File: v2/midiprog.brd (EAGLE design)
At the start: 99.1 x 78.7 mm, 56 parts, among them IC1 PIC18F4550_40, IC2 TPIC6B596N, IC4 TPIC6B596N, Q2 2N2222A, Q3 2N2222A, Q4 2N2222A, Q5 8MHz

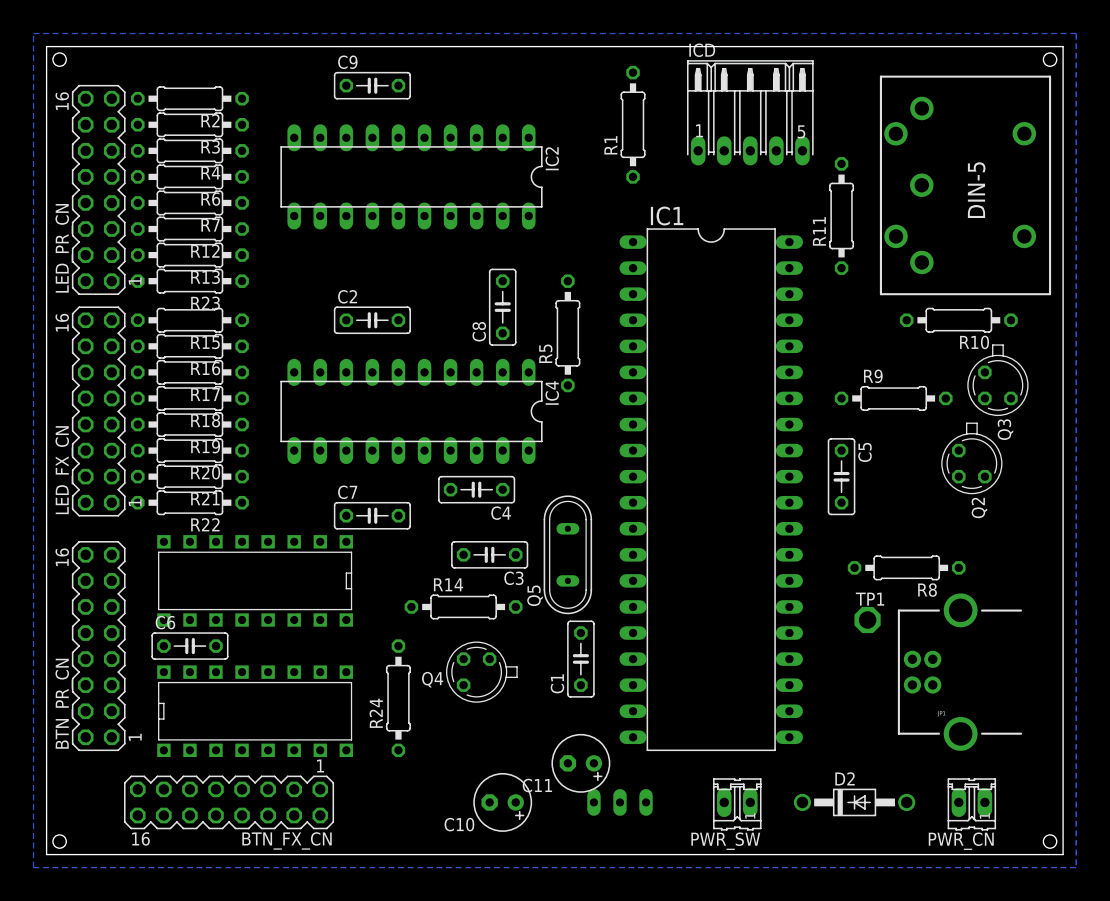
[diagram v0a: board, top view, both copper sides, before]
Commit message: Cleaning up board.
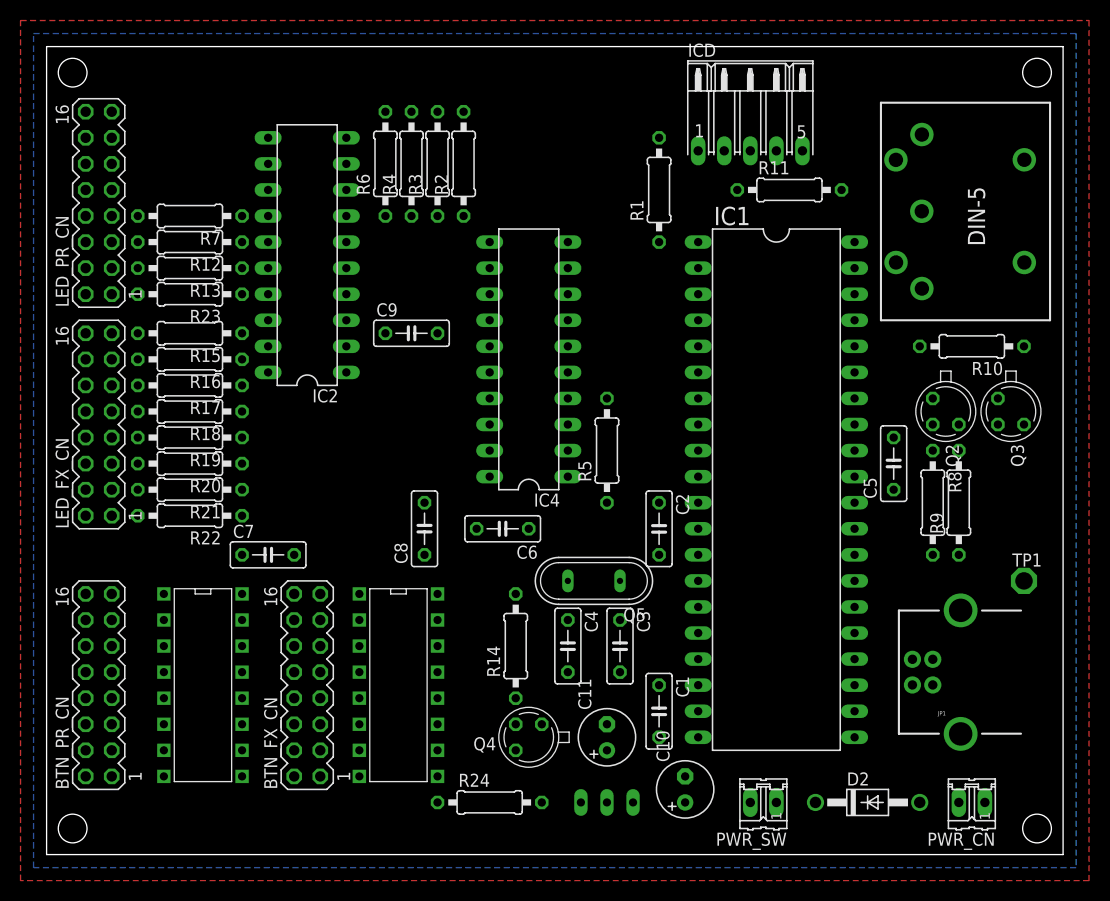
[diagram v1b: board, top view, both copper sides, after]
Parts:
- moved C2 34.5 mm to (59.7, 31.8), turned to 270 degrees
- moved C6 32.6 mm to (44.5, 31.8), turned to 180 degrees
- moved R2 27.4 mm to (40.6, 67.3), turned to 90 degrees
- moved C9 24.4 mm to (35.6, 50.8)
- moved R3 24.4 mm to (38.1, 67.3), turned to 90 degrees
- moved C8 22.9 mm to (36.8, 31.8)
- moved R4 21.6 mm to (35.6, 67.3), turned to 90 degrees
- moved R6 19.1 mm to (33.0, 67.3), turned to 90 degrees
- moved C10 17.8 mm to (62.2, 6.35), turned to 90 degrees
- moved C4 17.6 mm to (50.8, 20.3), turned to 270 degrees
- moved U$2 16.7 mm to (38.1, 15.2), turned to 270 degrees
- moved TP1 15.7 mm to (95.2, 26.7)
- moved C3 15.5 mm to (55.9, 20.3), turned to 270 degrees
- moved BTN_FX_CN 13.7 mm to (25.4, 16.5), turned to 90 degrees
- moved R24 13.5 mm to (43.2, 5.08), turned to 0 degrees
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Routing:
- added copper zone on layer 1, net GND
